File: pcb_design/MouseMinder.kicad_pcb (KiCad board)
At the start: 2 copper layers, 25.4 x 38.1 mm, 24 parts, among them J1 Conn_02x04_Odd_Even, Q1 SSM6L61NU,LF, SW1 SW_Push_Shielded, SW2 SW_Push_Shielded, U1 ATtiny10-TS

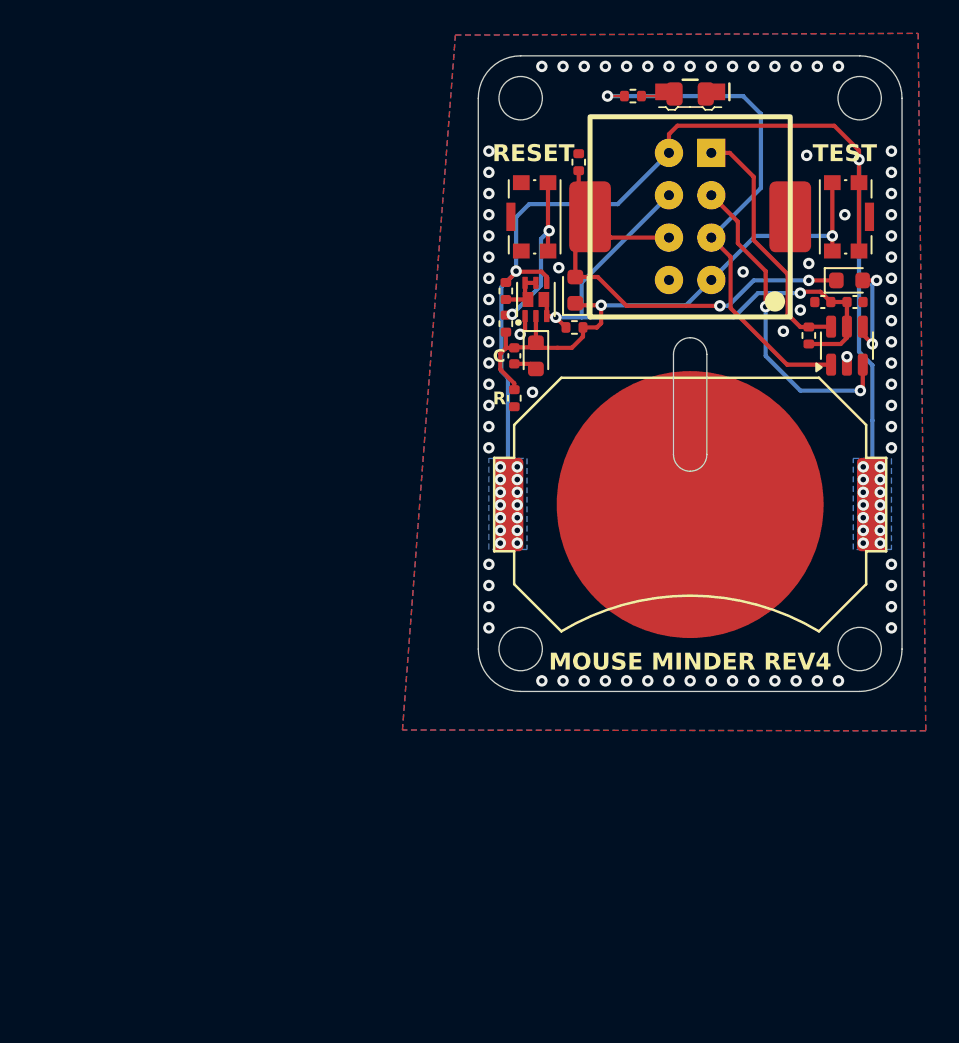
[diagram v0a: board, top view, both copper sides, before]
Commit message: Latest and cost-optimized!
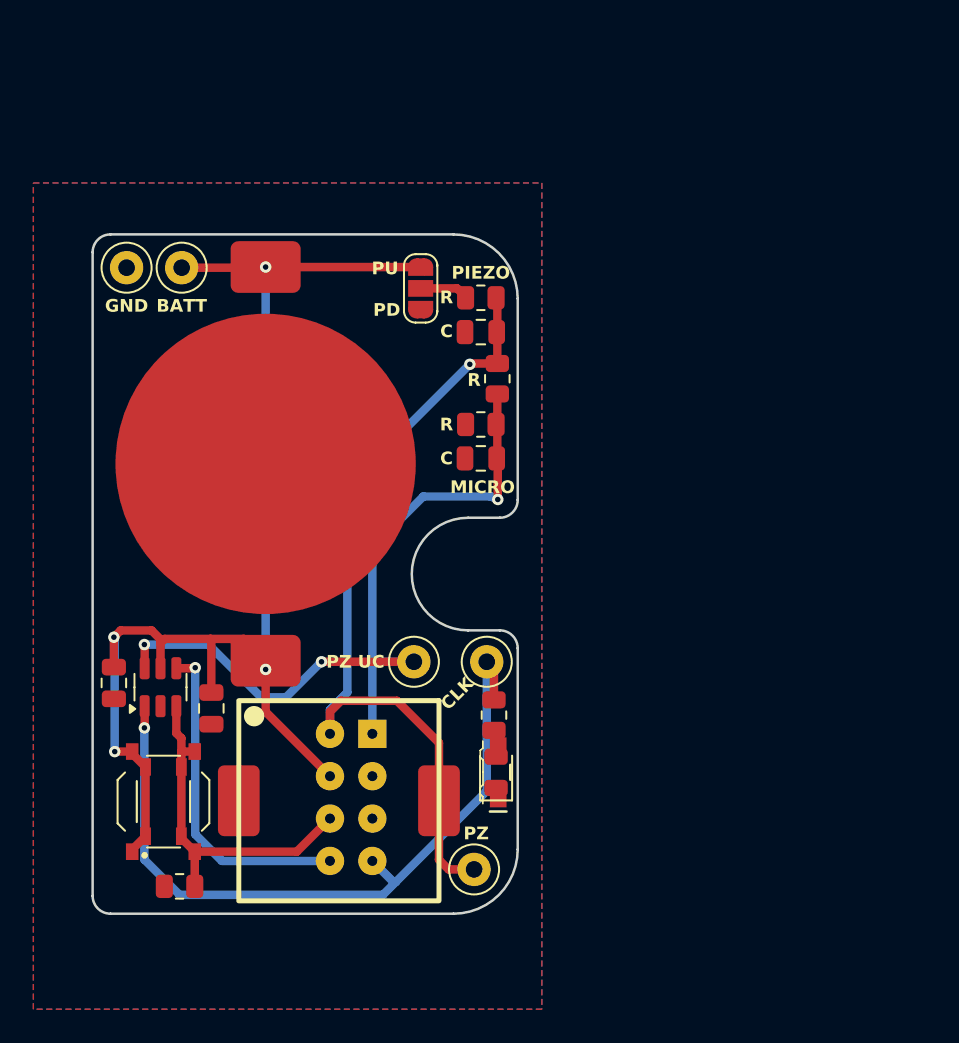
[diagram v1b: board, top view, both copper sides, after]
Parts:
- removed D3, D4: Schottky, Diode_SMD:D_0603_1608Metric
- removed D5: 2.7v, Diode_SMD:D_0603_1608Metric
- removed the G*** at (-6.86, -2.03)
- removed Q1: SSM6L61NU,LF, 0conrads:SON65P200X200X80-8N
- removed the R3 at (-10.5, 1.47)
- removed R6: 1k, Resistor_SMD:R_0402_1005Metric
- removed R7: 10k, Resistor_SMD:R_0402_1005Metric
- removed REF**: OSHW-Logo_5.7x6mm_SilkScreen, Symbol:OSHW-Logo_5.7x6mm_SilkScreen
- added C4: 100n, Capacitor_SMD:C_0805_2012Metric, F.Cu at (-34.5, 18.5)
- added G***: LOGO, 0art:mouseminder, B.Cu at (-25.9, 8.36)
- added JP1: SolderJumper_3_Open, Jumper:SolderJumper-3_P1.3mm_Open_RoundedPad1.0x1.5mm_NumberLabels, F.Cu at (-16.2, -5.11)
- added R1: 100k, Resistor_SMD:R_0805_2012Metric, F.Cu at (-12.5, -4.55)
- added TP1: TestPoint, TestPoint:TestPoint_Loop_D2.50mm_Drill1.0mm, F.Cu at (-30.5, -6.35)
- added TP2: TestPoint, TestPoint:TestPoint_Loop_D2.50mm_Drill1.0mm, F.Cu at (-33.8, -6.35)
- added TP3: TestPoint, TestPoint:TestPoint_Loop_D2.50mm_Drill1.0mm, F.Cu at (-13.0, 29.7)
- added TP4: TestPoint, TestPoint:TestPoint_Loop_D2.50mm_Drill1.0mm, F.Cu at (-16.6, 17.3)
- added TP5: TestPoint, TestPoint:TestPoint_Loop_D2.50mm_Drill1.0mm, F.Cu at (-12.2, 17.3)
- BT1: footprint 0conrads:MY-2032-08 -> 0conrads:C70373
- C1: value 10n -> 1u; footprint Capacitor_SMD:C_0402_1005Metric -> Capacitor_SMD:C_0805_2012Metric
- C2: footprint Capacitor_SMD:C_0402_1005Metric -> Capacitor_SMD:C_0805_2012Metric
- C3: value 100n -> 1u; footprint Capacitor_SMD:C_0402_1005Metric -> Capacitor_SMD:C_0805_2012Metric
- R2: value 1k -> 100; footprint Resistor_SMD:R_0402_1005Metric -> Resistor_SMD:R_0805_2012Metric
- R3: renamed from R1; footprint Resistor_SMD:R_0402_1005Metric -> Resistor_SMD:R_0805_2012Metric
- R4: value 10k -> 100k; footprint Resistor_SMD:R_0402_1005Metric -> Resistor_SMD:R_0805_2012Metric
- R5: value 10k -> 100; footprint Resistor_SMD:R_0402_1005Metric -> Resistor_SMD:R_0805_2012Metric
- SW1: value SW_Push_Shielded -> LCK-TA022H18-2WL; footprint Button_Switch_SMD:SW_Push_1P1T-SH_NO_CK_KMR2xxG -> Button_Switch_SMD:SW_Push_1P1T_XKB_TS-1187A
- SW2: value SW_Push_Shielded -> SKRPABE010; footprint Button_Switch_SMD:SW_Push_1P1T-SH_NO_CK_KMR2xxG -> 0conrads:SKRPABE010
- U1: value ATtiny10-TS -> PMS150C
- moved SW1 53.9 mm to (-31.6, 25.7), turned to 90 degrees
- moved U1 46.0 mm to (-31.8, 18.8)
- moved C3 45.6 mm to (-28.7, 20.1), turned to -90 degrees
- moved D1 42.3 mm to (-11.6, 23.9), turned to 90 degrees
- moved D2 42.3 mm to (-11.6, 23.9), turned to 90 degrees
- moved SW2 41.5 mm to (-31.6, 25.7)
- moved R4 41.0 mm to (-30.6, 30.7), turned to 180 degrees
- moved BZ1 40.8 mm to (-21.1, 25.6), turned to -90 degrees
- moved J3 40.3 mm to (-19.1, 21.6)
- moved R3 38.0 mm to (-11.8, 20.5), turned to -90 degrees
- moved BT1 25.6 mm to (-25.4, 5.41), turned to -90 degrees
- moved C2 22.5 mm to (-12.5, 5.08)
- moved R5 20.4 mm to (-12.5, 3.05), turned to 0 degrees
- moved R2 13.9 mm to (-11.6, 0.30)
- moved C1 2.46 mm to (-12.5, -2.49), turned to 180 degrees
- renumbered J1 to J3
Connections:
- BZ1 pad 1: PZ+ -> PIEZO
- C1 pad 1: NGATE -> PIEZO
- C2 pad 1: LATCHED_POWER -> PIEZO_UC
- C3 pad 1: LATCHED_POWER -> +3V0
- J3 pad 1: ~{RST} -> PIEZO_UC
- J3 pad 2: +3V0 -> PIEZO
- J3 pad 3: TPICLK -> GND
- J3 pad 4: LATCHED_POWER -> +3V0
- J3 pad 5: DATA -> unconnected-(J3-Pin_5-Pad5)
- J3 pad 6: PZ+ -> PROGMODE
- J3 pad 7: NGATE -> CLK
- J3 pad 8: GND -> HVPROG
- R2 pad 1: PZ+ -> PIEZO_UC
- R2 pad 2: GND -> PIEZO
- R3 pad 1: DATA -> CLK
- R4 pad 1: LATCHED_POWER -> PROGMODE
- R4 pad 2: NGATE -> GND
- R5 pad 1: LATCHED_POWER -> GND
- R5 pad 2: ~{RST} -> PIEZO_UC
- SW1 pad 2: NGATE -> PROGMODE
- SW2 pad 1: GND -> +3V0
- SW2 pad 2: Net-(R6-Pad2) -> PROGMODE
- U1 pad 1: DATA -> CLK
- U1 pad 3: TPICLK -> PROGMODE
- U1 pad 4: BUZZER -> HVPROG
- U1 pad 5: LATCHED_POWER -> +3V0
- U1 pad 6: ~{RST} -> PIEZO_UC
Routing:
- net PIEZO: track 0.00 -> 50.5 mm, vias 0 -> 1
- net PIEZO_UC: track 0.00 -> 48.7 mm, vias 0 -> 3
- net CLK: track 0.00 -> 45.3 mm, vias 0 -> 1
- net LATCHED_POWER: track 34.9 -> 0.00 mm, vias 2 -> 0
- net NGATE: track 34.8 -> 0.00 mm, vias 2 -> 0
- net DATA: track 31.4 -> 0.00 mm, vias 1 -> 0
- net PZ+: track 29.3 -> 0.00 mm, vias 2 -> 0
- net PROGMODE: track 0.00 -> 21.0 mm
- net HVPROG: track 0.00 -> 19.9 mm, vias 0 -> 1
- net TPICLK: track 19.1 -> 0.00 mm, vias 2 -> 0
- net ~{RST}: track 15.1 -> 0.00 mm
- net Net-(R6-Pad2): track 10.5 -> 0.00 mm, vias 2 -> 0
- net BUZZER: track 6.03 -> 0.00 mm, vias 2 -> 0
- net +3V0: track 73.2 -> 79.0 mm, vias 30 -> 4
- net /PGATE: track 3.05 -> 0.00 mm
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- removed copper zone on B.Cu, net +3V0
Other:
- board size 25.4 x 38.1 mm -> 25.5 x 40.7 mm
- board text added: "BATT"
- board text added: "HVPROG"
- board text added: "MICRO"
- board text added: "NC"
- board text added: "PD"
- board text added: "PIEZO"
- board text added: "PROGMODE"
- board text added: "PU"
- board text added: "PZ UC"
- board text added: "REVISION 5 JUL. 2026"
- board text added: "TO DO: Fix Pogo Programmer Holes!"
- board text added: "WWW.MOUSEMINDER.COM"
- board text removed: "BATTERY: CR2032"
- board text removed: "DATA"
- board text removed: "LATCHED"
- board text removed: "MOUSE MINDER REV4"
- board text removed: "NGATE"
- board text removed: "PEN OR SOMETHING"
- board text removed: "RESET"
- board text removed: "TEST"
- board text removed: "WWW.FARNSWORTH.ENGINEERING"
- board text removed: "~{RST}"
